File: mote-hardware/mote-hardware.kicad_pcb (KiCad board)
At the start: 2 copper layers, 93.6 x 102.8 mm, 67 parts, among them J1 USB_C_Receptacle_USB2.0_14P, J2 JST_XH2.54-SP, J4 SM03B-SRSS-TB, J5 Conn_01x03_Pin, J6 Conn_01x03_Pin, J7 JST_PH_B6B, J8 JST_PH_B6B, SW1 SW_Push, SW2 SW_Push, U1 RP2354_60QFN, U2 NCP1117-3.3_SOT223, U4 RP Radio Module 2, U5 DRV8833PW, U9 LSM6DS3, Y1 ABM8-272-T3

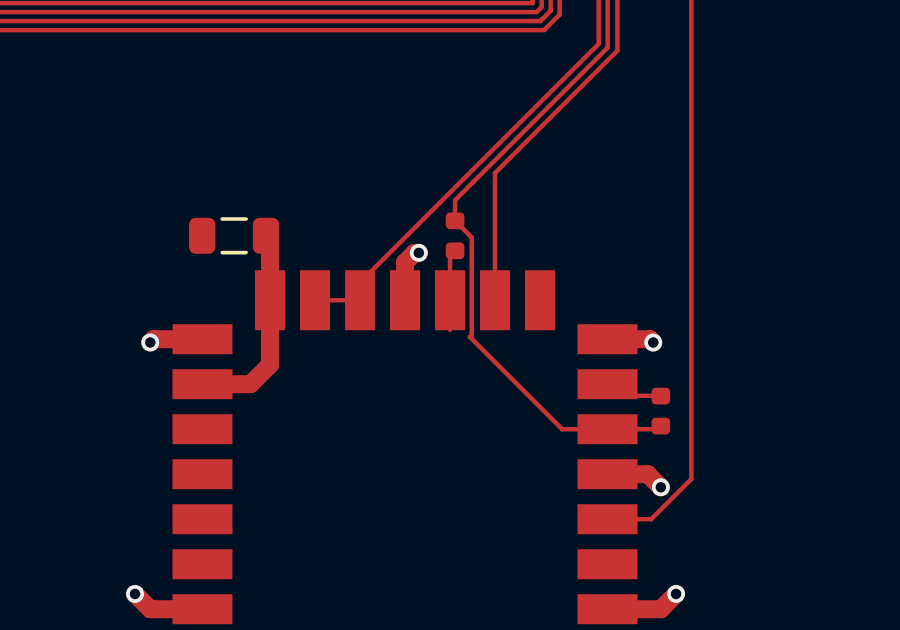
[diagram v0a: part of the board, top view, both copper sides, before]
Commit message: mend
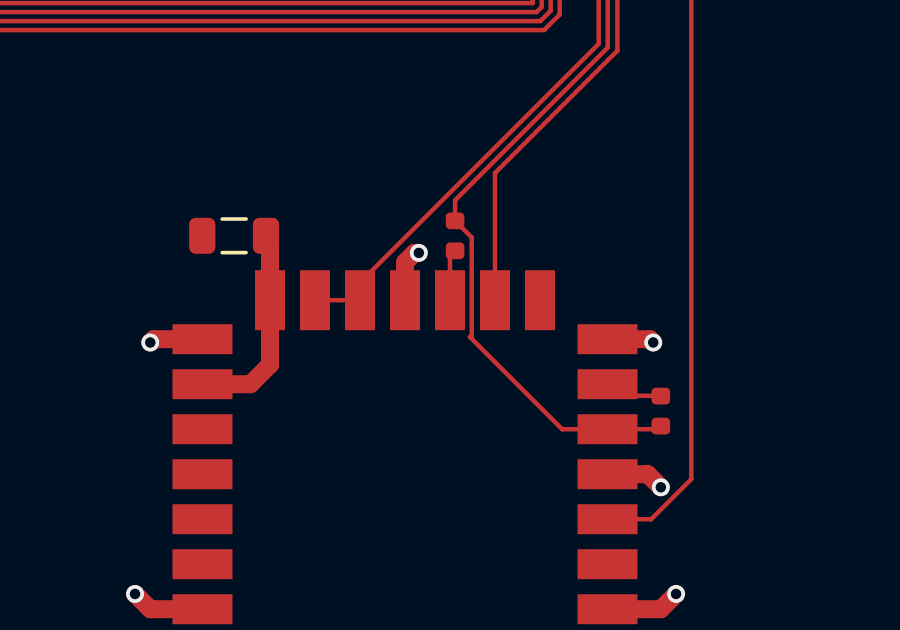
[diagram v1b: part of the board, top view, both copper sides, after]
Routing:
- net Net-(U4-nIRQ): track 2.70 -> 1.72 mm
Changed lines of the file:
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@@
-	)
-	(segment
-		(start 101.43 126.098)
-		(end 101.43 127.084)
-		(width 0.15)
-		(layer "F.Cu")
-		(net 39)
 	)
 	(segment
